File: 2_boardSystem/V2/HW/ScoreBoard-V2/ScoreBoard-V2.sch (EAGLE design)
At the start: 47 parts, among them M1 VNH5019, M2 VNH5019, M3 VNH5019, M4 VNH5019, M5 VNH5019, M6 VNH5019, U1 TXB0108

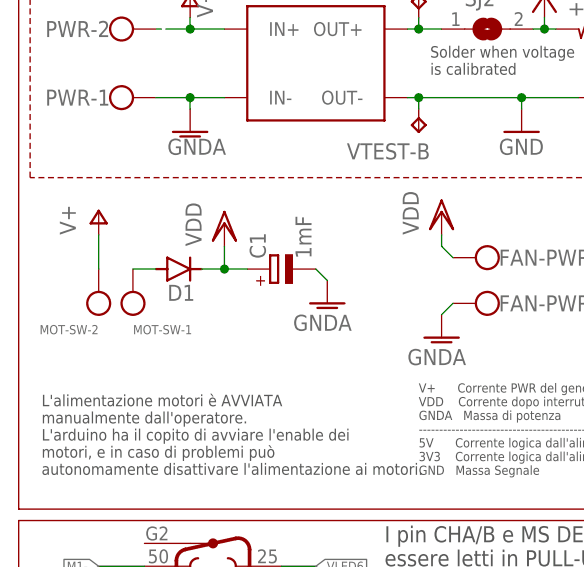
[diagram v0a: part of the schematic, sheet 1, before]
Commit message: ScorBoard-manual-V2
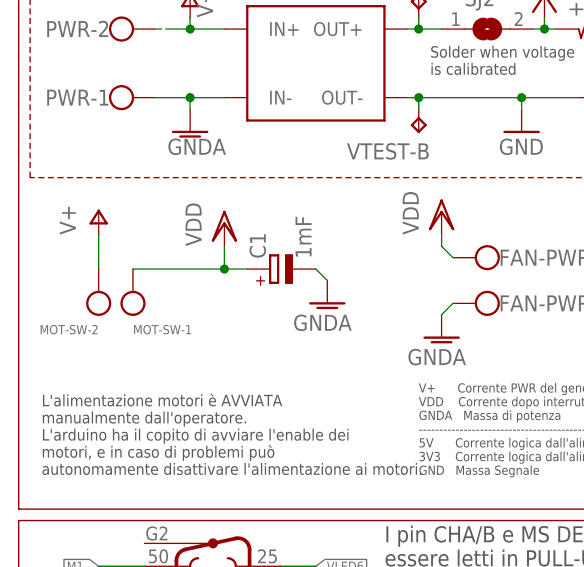
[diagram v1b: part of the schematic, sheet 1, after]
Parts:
- removed D1: ES2D, diode:ES2D
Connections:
- removed net N$2: D1.A, MOT-SW-1.KL
- net VDD: now also MOT-SW-1.KL; no longer D1.C
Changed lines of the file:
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@@
 <part name="U$1" library="loghi" deviceset="ALFY-BIG" device=""/>
 <part name="U$4" library="loghi" deviceset="ALFY-BIG" device=""/>
-<part name="D1" library="diode" library_urn="urn:adsk.eagle:library:210" deviceset="ES2D" device="" package3d_urn="urn:adsk.eagle:package:43404/2"/>
 <part name="V-OFF-PAD" library="testpad" deviceset="TP2" device="P2-38-17" package3d_urn="urn:adsk.eagle:package:27945/1">
 <attribute name="SPICEPREFIX" value="X"/>
@@
 </instance>
 <instance part="U$1" gate="G$1" x="10.16" y="15.24" smashed="yes"/>
-<instance part="D1" gate="G$1" x="22.86" y="138.43" smashed="yes" rot="MR180">
-<attribute name="NAME" x="21.59" y="136.6774" size="1.778" layer="95" rot="MR180"/>
-</instance>
 <instance part="V-OFF-PAD" gate="A" x="233.68" y="167.64" smashed="yes">
 <attribute name="NAME" x="224.79" y="168.91" size="1.778" layer="95"/>
@@
 <pinref part="C1" gate="G$1" pin="+"/>
 <wire x1="27.94" y1="138.43" x2="30.48" y2="138.43" width="0.1524" layer="91"/>
-<pinref part="D1" gate="G$1" pin="C"/>
-<wire x1="25.4" y1="138.43" x2="27.94" y2="138.43" width="0.1524" layer="91"/>
 <junction x="27.94" y="138.43"/>
+<pinref part="MOT-SW" gate="-1" pin="KL"/>
+<wire x1="17.78" y1="138.43" x2="27.94" y2="138.43" width="0.1524" layer="91"/>
 </segment>
 <segment>
@@
 </segment>
 </net>
-<net name="N$2" class="1">
-<segment>
-<pinref part="D1" gate="G$1" pin="A"/>
-<pinref part="MOT-SW" gate="-1" pin="KL"/>
-<wire x1="20.32" y1="138.43" x2="17.78" y2="138.43" width="0.1524" layer="91"/>
-</segment>
-</net>
